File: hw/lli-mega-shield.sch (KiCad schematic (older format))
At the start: 33 parts, among them K1 36.11.9.003.4000, P1 Enable, P3 AUX A, P4 AUX B, Q1 NPN, U1 APC220, U2 LM35, U3 LM35, U4 LM35, U5 ADIS16405, U6 R-78B5.0-1.5

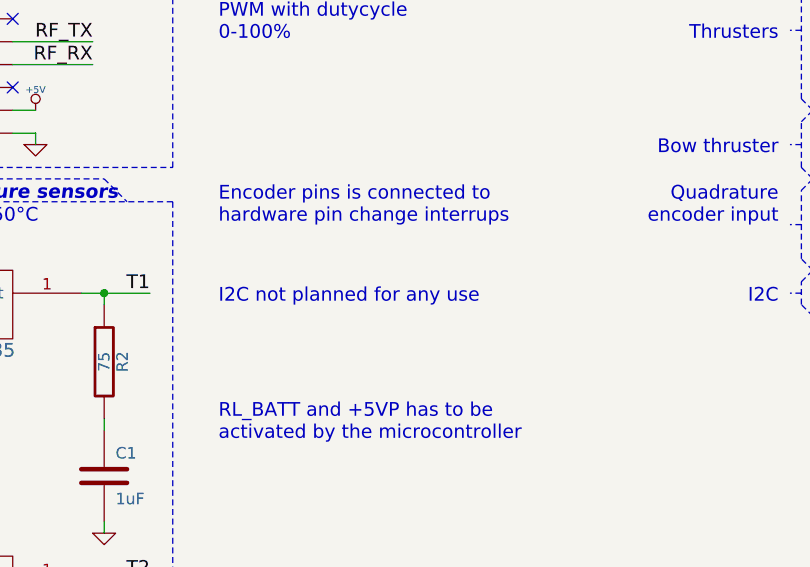
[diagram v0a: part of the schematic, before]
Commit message: Some updates to hw
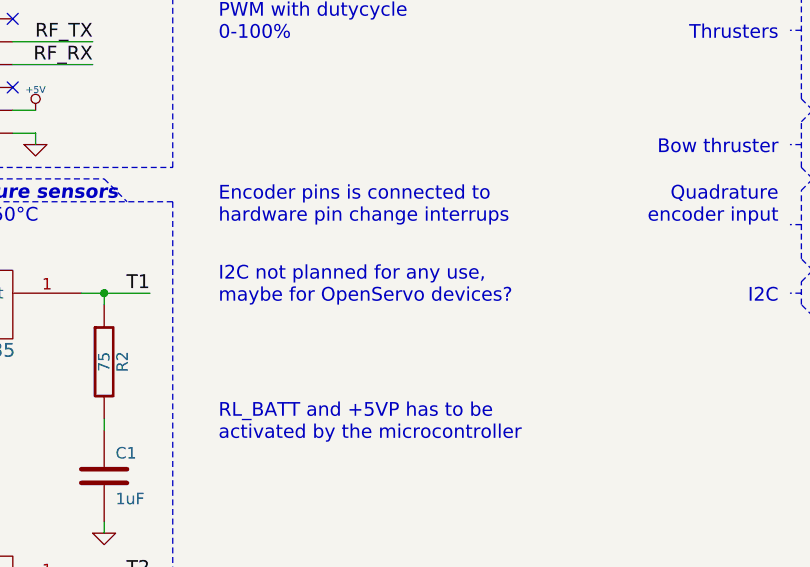
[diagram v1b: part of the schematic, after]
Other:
- note added: "I2C not planned for any use,\nmaybe for OpenServo devices?"
- note removed: "I2C not planned for any use"
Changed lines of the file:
@@
-EESchema Schematic File Version 2  date søn 23 sep 2012 11:40:33 CEST
+EESchema Schematic File Version 2  date søn 23 sep 2012 12:03:57 CEST
 LIBS:power
 LIBS:device
@@
 RL_BATT
 Text Notes 2400 2350 0    60   ~ 0
-I2C not planned for any use
+I2C not planned for any use,\nmaybe for OpenServo devices?
 Text Notes 4850 2350 2    60   ~ 0
 I2C
